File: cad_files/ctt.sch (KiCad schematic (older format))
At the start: 5 parts, among them CN1 CONN_3, CN2 CONN_3, J1 RELAY

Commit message: 220902
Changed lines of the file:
@@
-EESchema Schematic File Version 2  date 2012.01.28. 6:39:46
+EESchema Schematic File Version 2
+LIBS:ctt-rescue
 LIBS:power
 LIBS:device
@@
 LIBS:memory
 LIBS:xilinx
-LIBS:special
 LIBS:microcontrollers
 LIBS:dsp
@@
 LIBS:valves
 LIBS:ctt-cache
-EELAYER 24  0
+EELAYER 25 0
 EELAYER END
-$Descr A4 11700 8267
+$Descr A4 11693 8268
+encoding utf-8
 Sheet 1 11
 Title "CTT Transistor tester"
@@
 F 0 "J1" H 2000 7500 60  0000 C CNN
 F 1 "RELAY" H 1850 7175 60  0001 C CNN
+F 2 "" H 1825 7400 60  0001 C CNN
+F 3 "" H 1825 7400 60  0001 C CNN
 	1    1825 7400
 	1    0    0    -1
@@
 26
 $Comp
-L GND #PWR?
+L GND-RESCUE-ctt #PWR?
 U 1 1 4DEB2E58
 P 975 5150
 F 0 "#PWR?" H 975 5150 30  0001 C CNN
 F 1 "GND" H 975 5080 30  0001 C CNN
+F 2 "" H 975 5150 60  0001 C CNN
+F 3 "" H 975 5150 60  0001 C CNN
 	1    975  5150
 	1    0    0    -1
@@
 CN1
 $Comp
-L GND #PWR?
+L GND-RESCUE-ctt #PWR?
 U 1 1 4DD14509
 P 8750 6700
 F 0 "#PWR?" H 8750 6700 30  0001 C CNN
 F 1 "GND" H 8750 6630 30  0001 C CNN
+F 2 "" H 8750 6700 60  0001 C CNN
+F 3 "" H 8750 6700 60  0001 C CNN
 	1    8750 6700
 	1    0    0    -1
@@
 F 0 "JC1" H 1625 5625 50  0000 C CNN
 F 1 "SWITCH_INV" H 1725 5625 50  0001 C CNN
+F 2 "" H 1875 5775 60  0001 C CNN
+F 3 "" H 1875 5775 60  0001 C CNN
 	1    1875 5775
 	-1   0    0    1
@@
 F 0 "JC2" H 1625 6300 50  0000 C CNN
 F 1 "SWITCH_INV" H 1725 6000 50  0001 C CNN
+F 2 "" H 1875 6150 60  0001 C CNN
+F 3 "" H 1875 6150 60  0001 C CNN
 	1    1875 6150
 	-1   0    0    -1
@@
 27
 $Comp
-L GND #PWR?
+L GND-RESCUE-ctt #PWR?
 U 1 1 4DCFFEB2
 P 4675 6825
 F 0 "#PWR?" H 4675 6825 30  0001 C CNN
 F 1 "GND" H 4675 6755 30  0001 C CNN
+F 2 "" H 4675 6825 60  0001 C CNN
+F 3 "" H 4675 6825 60  0001 C CNN
 	1    4675 6825
 	1    0    0    -1
@@
 F 0 "CN2" V 6650 1900 50  0000 C CNN
 F 1 "CONN_3" V 6750 1900 40  0001 C CNN
+F 2 "" H 6700 1900 60  0001 C CNN
+F 3 "" H 6700 1900 60  0001 C CNN
 	1    6700 1900
 	1    0    0    -1
@@
 F 0 "#PWR?" H 8950 6750 40  0001 C CNN
 F 1 "GNDPWR" V 8950 6500 40  0001 C CNN
+F 2 "" H 8950 6700 60  0001 C CNN
+F 3 "" H 8950 6700 60  0001 C CNN
 	1    8950 6700
 	1    0    0    -1
@@
 F 0 "CN1" V 10800 4550 50  0000 C CNN
 F 1 "CONN_3" V 10900 4550 40  0001 C CNN
+F 2 "" H 10850 4550 60  0001 C CNN
+F 3 "" H 10850 4550 60  0001 C CNN
 	1    10850 4550
 	1    0    0    -1
@@
 26
 $Comp
-L GND #PWR?
+L GND-RESCUE-ctt #PWR?
 U 1 1 4D1605BF
 P 10750 2250
 F 0 "#PWR?" H 10750 2250 30  0001 C CNN
 F 1 "GND" H 10750 2180 30  0001 C CNN
+F 2 "" H 10750 2250 60  0001 C CNN
+F 3 "" H 10750 2250 60  0001 C CNN
 	1    10750 2250
 	1    0    0    -1
@@
 26
 $Comp
-L GND #PWR?
+L GND-RESCUE-ctt #PWR?
 U 1 1 4D1605B5
 P 8800 2250
 F 0 "#PWR?" H 8800 2250 30  0001 C CNN
 F 1 "GND" H 8800 2180 30  0001 C CNN
+F 2 "" H 8800 2250 60  0001 C CNN
+F 3 "" H 8800 2250 60  0001 C CNN
 	1    8800 2250
 	1    0    0    -1
 $EndComp
 $Comp
-L GND #PWR?
+L GND-RESCUE-ctt #PWR?
 U 1 1 4D1605A3
 P 7050 4900
 F 0 "#PWR?" H 7050 4900 30  0001 C CNN
 F 1 "GND" H 7050 4830 30  0001 C CNN
+F 2 "" H 7050 4900 60  0001 C CNN
+F 3 "" H 7050 4900 60  0001 C CNN
 	1    7050 4900
 	1    0    0    -1
@@
 24
 $Comp
-L GND #PWR?
+L GND-RESCUE-ctt #PWR?
 U 1 1 4D15FE06
 P 2850 2250
 F 0 "#PWR?" H 2850 2250 30  0001 C CNN
 F 1 "GND" H 2850 2180 30  0001 C CNN
+F 2 "" H 2850 2250 60  0001 C CNN
+F 3 "" H 2850 2250 60  0001 C CNN
 	1    2850 2250
 	1    0    0    -1

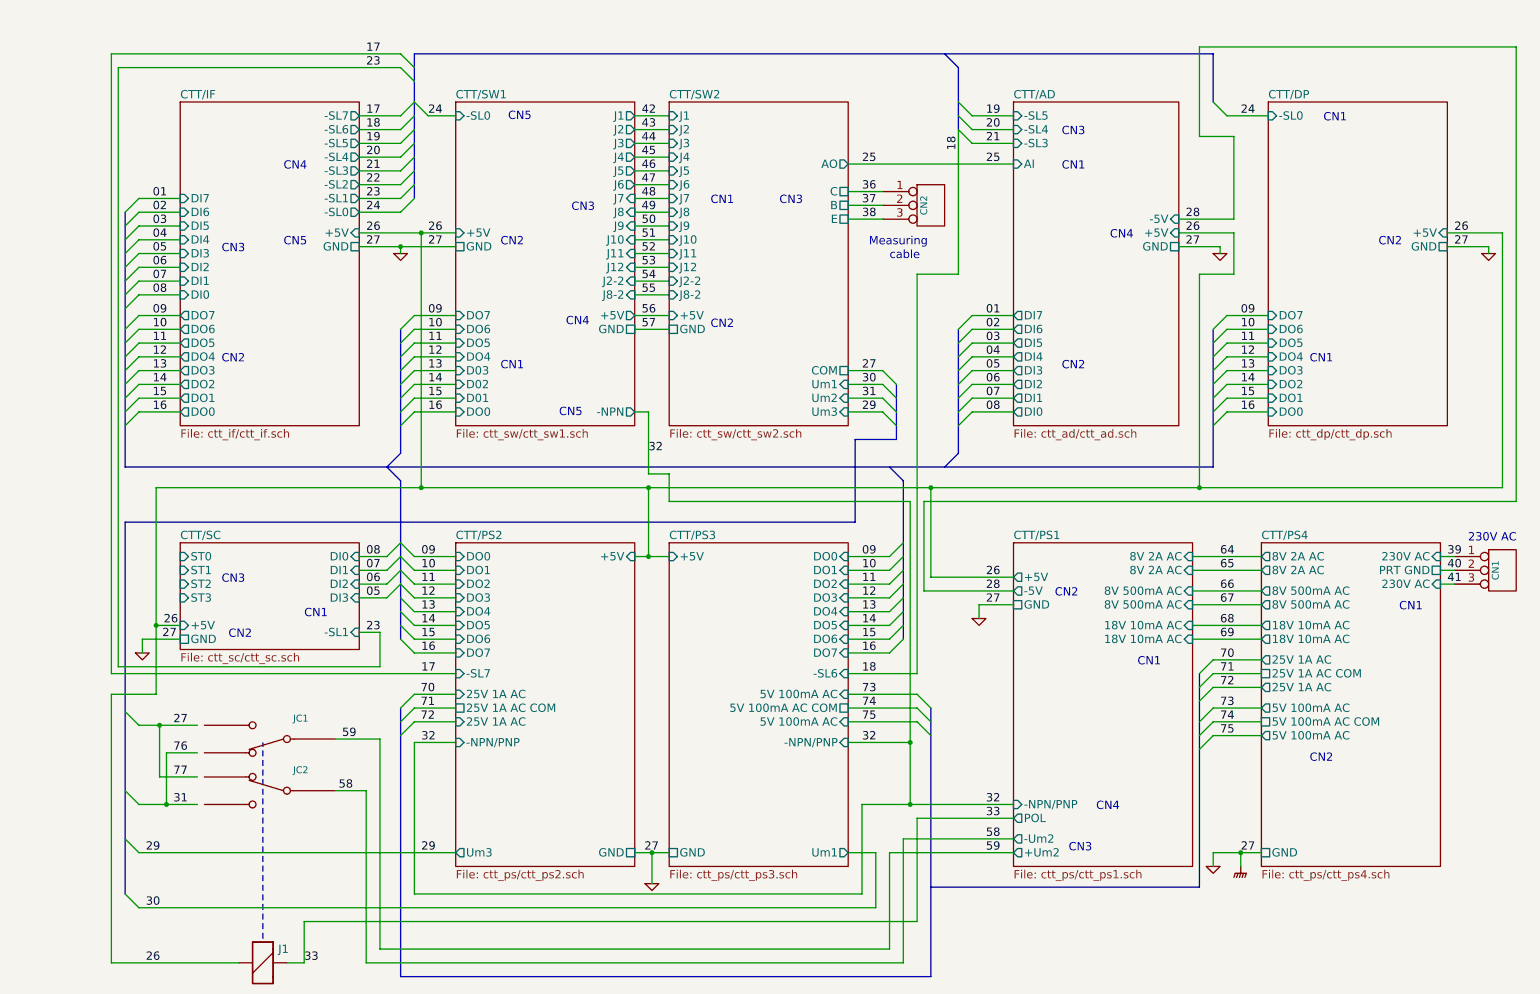
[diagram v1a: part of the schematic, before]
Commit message: 220903
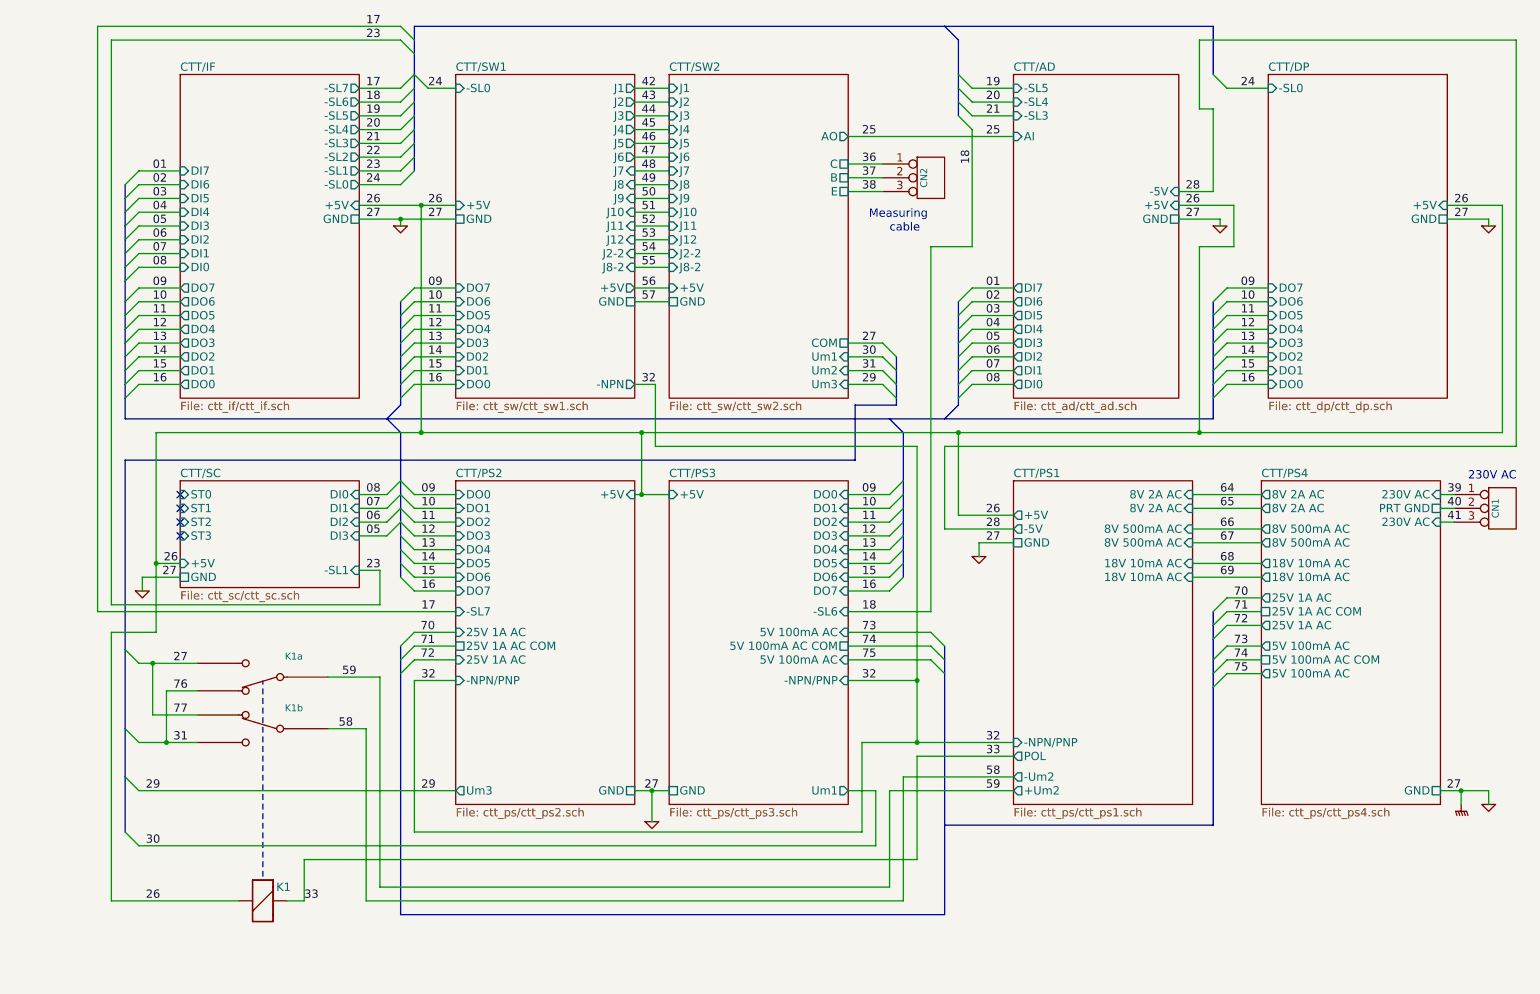
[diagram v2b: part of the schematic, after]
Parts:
- renumbered J1 to K1, JC1 to K1a, JC2 to K1b
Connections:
- net 31: now also K1a.1, K1b.3
- net GND: now also K1a.3, K1b.1
- no-connect marks 0 -> 4
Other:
- note removed: "CN1"
- note removed: "CN2"
- note removed: "CN3"
- note removed: "CN4"
- note removed: "CN5"
- moved on the sheet: CN1, CN2, K1, K1a, K1b

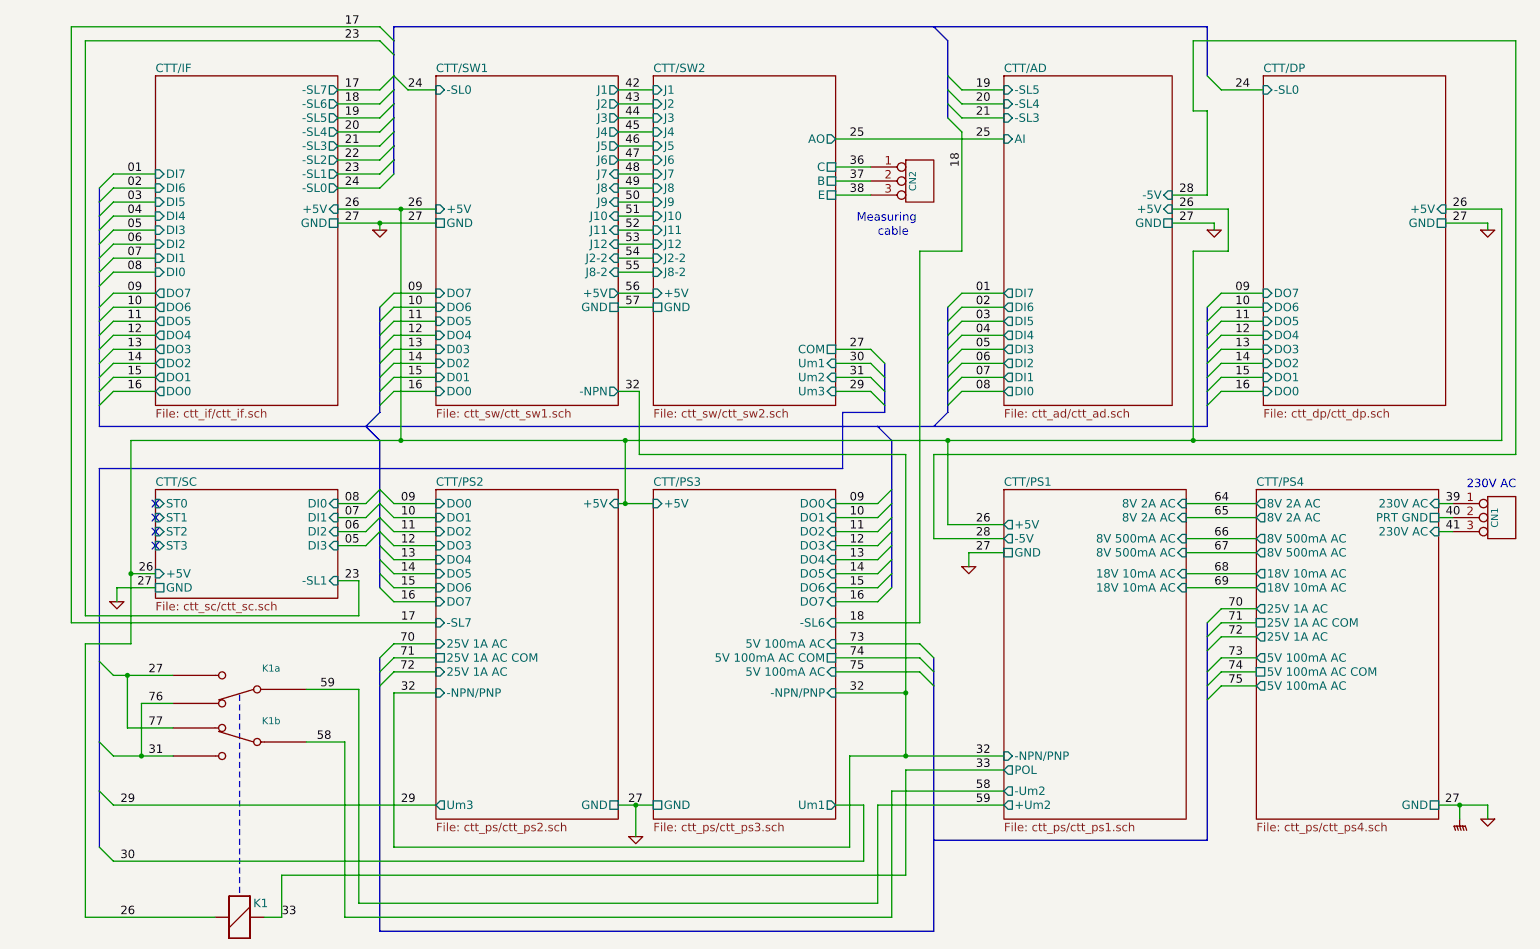
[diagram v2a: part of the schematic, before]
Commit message: 220905
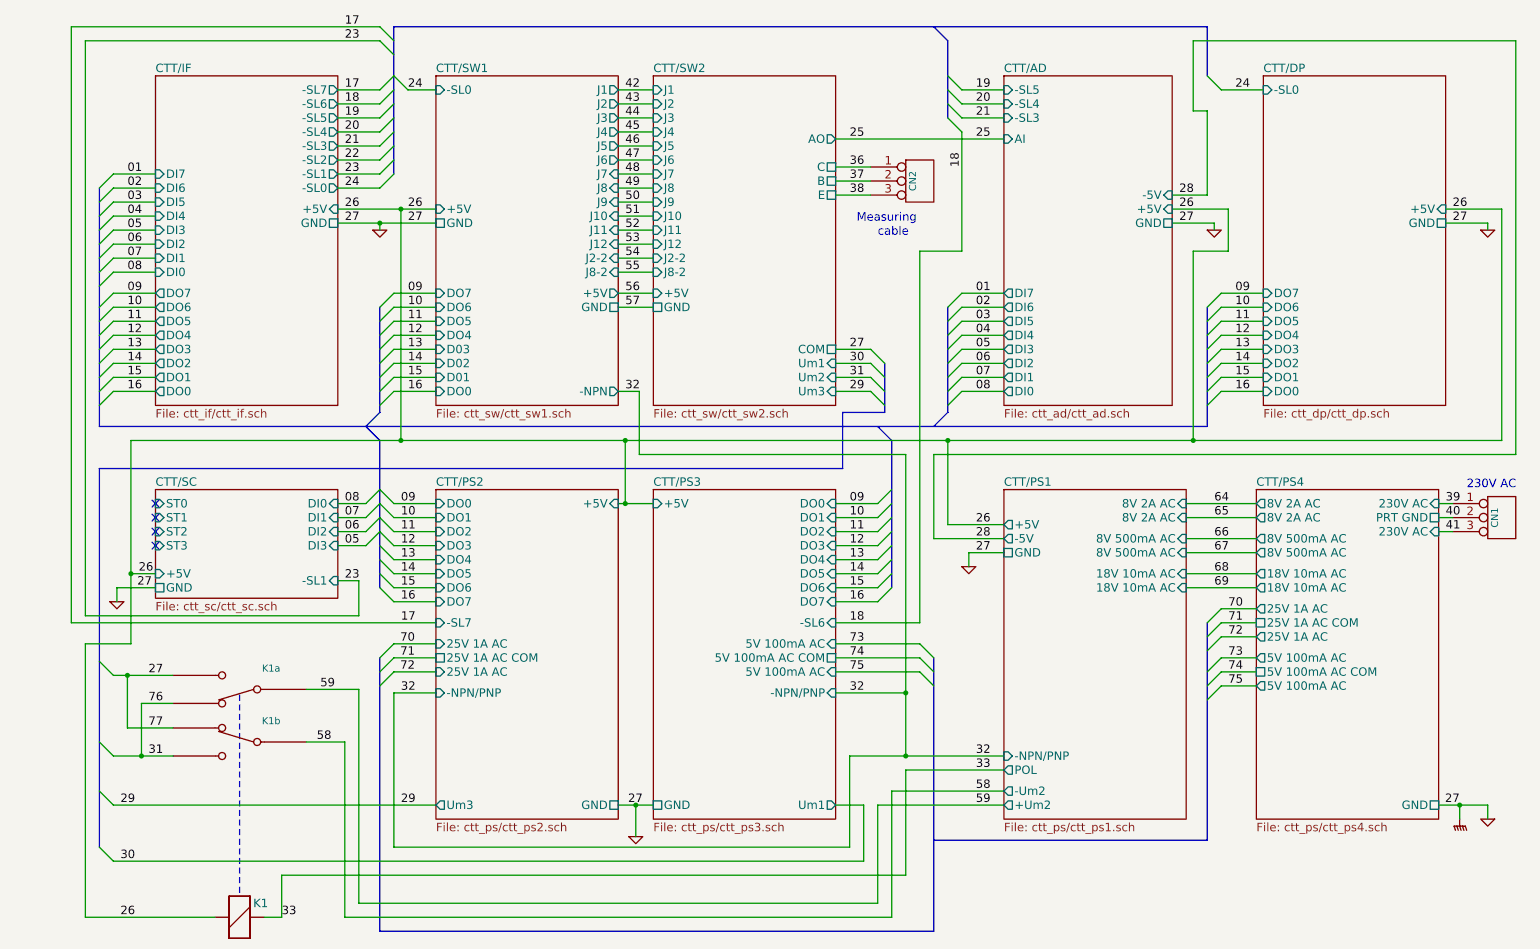
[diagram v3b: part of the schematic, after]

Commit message: 220907
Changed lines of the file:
@@
 	6800 7050 2850 7050
 Wire Bus Line
-	2850 5100 2850 7050
+	2850 7050 2850 5100
 Wire Wire Line
 	3250 5100 2950 5100

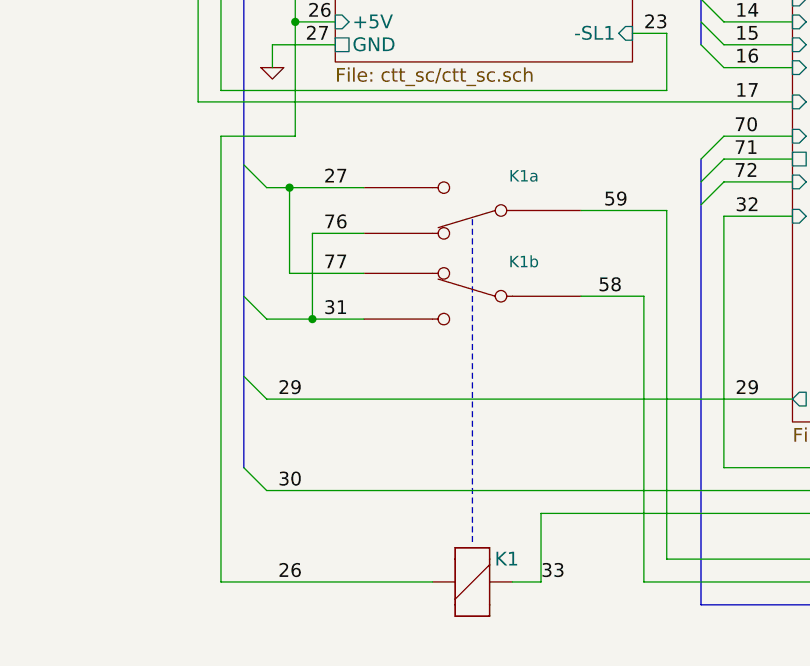
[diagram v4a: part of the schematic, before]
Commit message: 220911
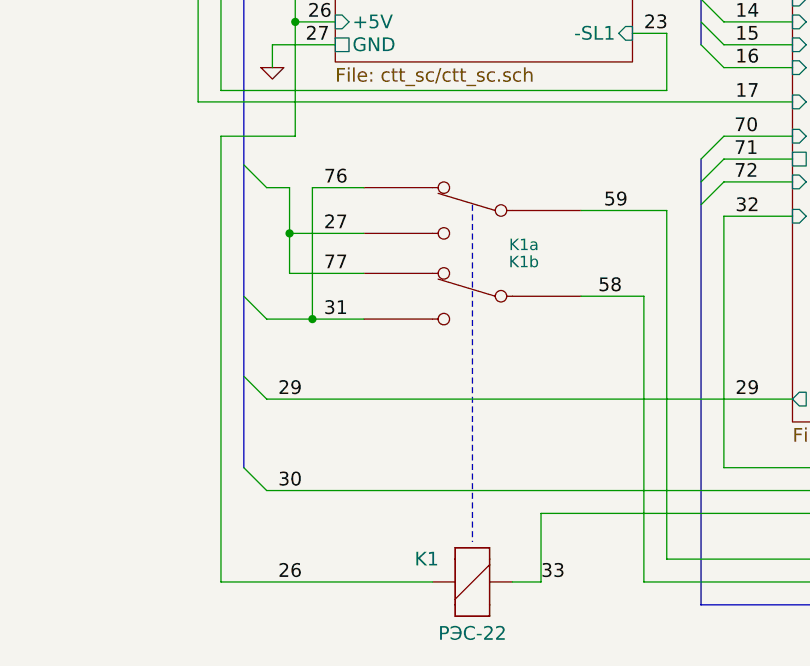
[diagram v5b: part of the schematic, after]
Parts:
- K1: value RELAY -> РЭС-22
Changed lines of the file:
@@
 Wire Wire Line
 	7300 5900 6600 5900
-Connection ~ 1050 5225
-Wire Wire Line
-	950  5225 1375 5225
+Wire Wire Line
+	1050 5425 1375 5425
 Wire Bus Line
 	6450 3000 6450 3350
 Wire Wire Line
 	6350 3100 6100 3100
-Wire Wire Line
-	1050 5225 1050 5600
 Wire Wire Line
 	1050 5600 1375 5600
@@
 	2600 5700 2325 5700
 Wire Wire Line
-	1375 5425 1150 5425
-Wire Wire Line
-	1150 5425 1150 5800
+	1375 5225 1150 5225
+Wire Wire Line
+	1150 5225 1150 5800
 Wire Wire Line
 	6100 3000 6350 3000
@@
 	750  6950 1675 6950
 Wire Notes Line
-	1850 6775 1850 5350
+	1850 5300 1850 6775
 Wire Wire Line
 	6300 6550 950  6550
@@
 U 1 1 4E2F1050
 P 1825 6950
-F 0 "K1" H 2000 7050 60  0000 C CNN
-F 1 "RELAY" H 1850 6725 60  0001 C CNN
+F 0 "K1" H 1650 7050 60  0000 C CNN
+F 1 "РЭС-22" H 1850 6725 60  0000 C CNN
 F 2 "" H 1825 6950 60  0001 C CNN
 F 3 "" H 1825 6950 60  0001 C CNN
@@
 Text Label 1200 5600 0    60   ~ 0
 77
-Text Label 1200 5425 0    60   ~ 0
+Text Label 1200 5225 0    60   ~ 0
 76
 Text Label 8900 5300 0    60   ~ 0
@@
 Text Label 8900 4750 0    60   ~ 0
 70
-Text Label 1200 5225 0    60   ~ 0
+Text Label 1200 5425 0    60   ~ 0
 27
 Text Label 1200 5800 0    60   ~ 0
@@
 F 3 "" H 1825 5325 60  0001 C CNN
 	1    1825 5325
-	-1   0    0    1
+	-1   0    0    -1
 $EndComp
 $Comp
@@
 F14 "POL" O L 7300 5900 60
 $EndSheet
+Wire Wire Line
+	1050 5225 1050 5600
+Wire Wire Line
+	1050 5225 950  5225
+Connection ~ 1050 5425
 $EndSCHEMATC
